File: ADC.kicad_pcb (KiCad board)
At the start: 2 copper layers, 199 parts, among them J1 Conn_01x03_Pin, J2 Screw_Terminal_01x02, J3 Screw_Terminal_01x09, SW1 SW_SPDT, U1 ADS1256IDBR, U10 CD4514BM, U11 ADG5412FBCPZ-RL7, U12 ADR421ARMZ, U13 OPA211ID, U14 ADG5412FBCPZ-RL7, U15 OPA211ID, U16 ADG5412FBCPZ-RL7, U17 OPA211ID, U18 CD4072BM, U19 CD4514BM, U2 MCU-STM32F407VET6_LQFP100_, U20 ADG5412FBCPZ-RL7, U21 ADG5412FBCPZ-RL7, U22 ADG5412FBCPZ-RL7, U23 ADG5412FBCPZ-RL7, U24 OPA211ID, U25 OPA211ID, U26 OPA211ID, U27 OPA211ID, U28 CD4043BPWR, U29 TLV1704AIPWR, U3 ADM2483xRW, U30 TLV1704AIPWR, U31 TLV1704AIPWR, U32 CD4072BM, U4 LM2596S-5, U5 DCP010505BP, U6 TLV1704AIPWR, U7 OPA211ID, U8 AMS1117-3.3, U9 ADG5412FBCPZ-RL7, Y1 8MHz, Y2 ABM3B-25.000MHZ-D2Y-T

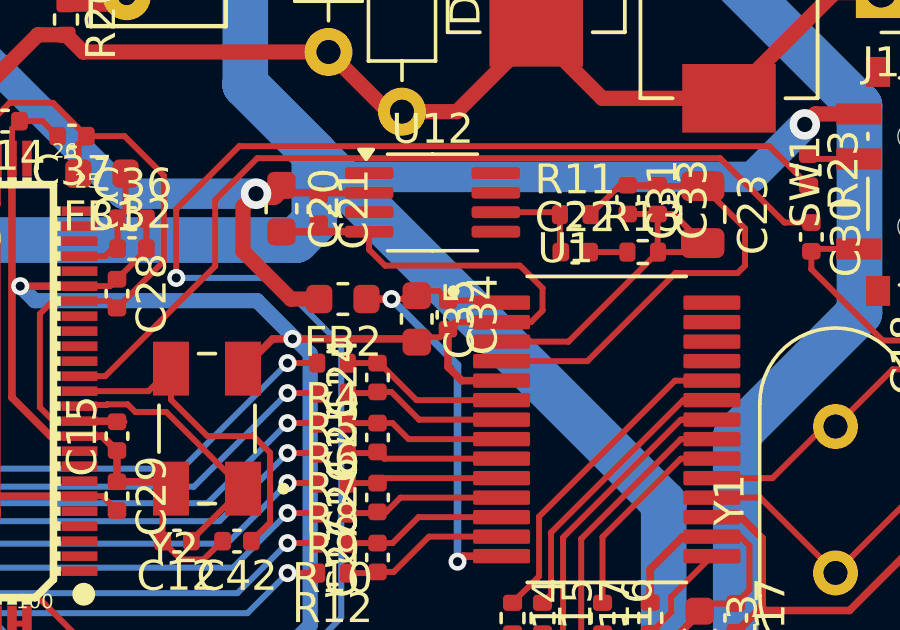
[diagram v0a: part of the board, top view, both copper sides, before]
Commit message: update
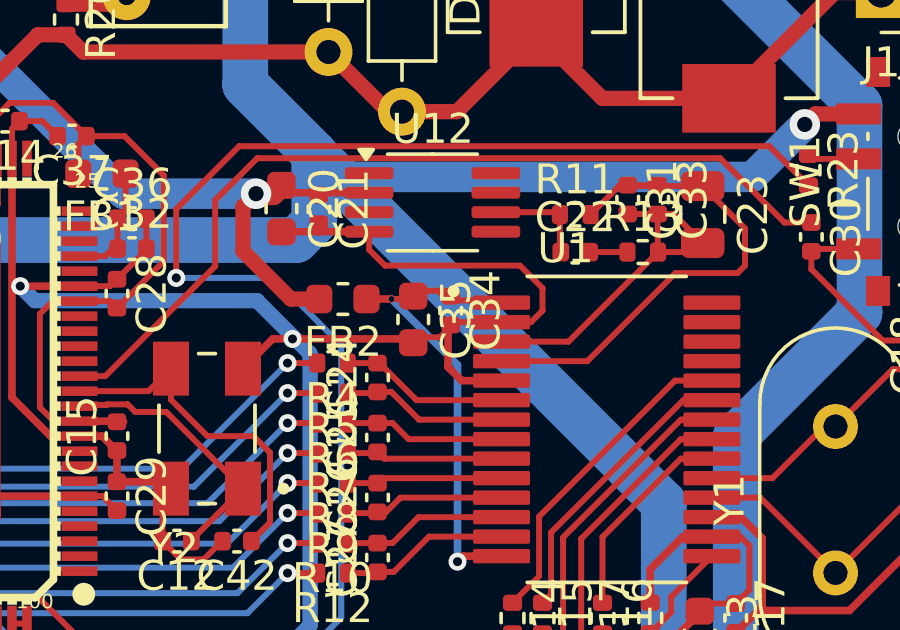
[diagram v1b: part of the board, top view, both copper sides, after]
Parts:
- moved C34 0.17 mm to (633.0, 474.1)
- moved C35 0.12 mm to (631.8, 474.4)
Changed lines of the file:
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@@
 		(tags "C Radial series Radial pin pitch 3.50mm diameter 8mm height 7mm Non-Polar Electrolytic Capacitor")
 		(property "Reference" "C4"
-			(at 1.75 -5.25 360)
+			(at 1.75 -5.25 0)
 			(layer "F.SilkS")
 			(effects
@@
 		)
 		(property "Value" "47uF"
-			(at 1.75 5.25 360)
+			(at 1.75 5.25 0)
 			(layer "F.Fab")
 			(effects
@@
 		)
 		(fp_text user "${REFERENCE}"
-			(at 1.75 0 360)
+			(at 1.75 0 0)
 			(layer "F.Fab")
 			(effects
@@
 		)
 		(fp_text user "${REFERENCE}"
-			(at 0 0 360)
+			(at 0 0 0)
 			(layer "F.Fab")
 			(effects
@@
 		(tags "C Radial series Radial pin pitch 3.50mm diameter 8mm height 7mm Non-Polar Electrolytic Capacitor")
 		(property "Reference" "C1"
-			(at 1.75 -5.25 360)
+			(at 1.75 -5.25 0)
 			(layer "F.SilkS")
 			(effects
@@
 		)
 		(property "Value" "47uF"
-			(at 1.75 5.25 360)
+			(at 1.75 5.25 0)
 			(layer "F.Fab")
 			(effects
@@
 		)
 		(fp_text user "${REFERENCE}"
-			(at 1.75 0 360)
+			(at 1.75 0 0)
 			(layer "F.Fab")
 			(effects
@@
 	(footprint "Capacitor_SMD:C_0402_1005Metric"
 		(layer "F.Cu")
-		(at 632.959137 474.220735 -90)
+		(at 633.05 474.08 -90)
 		(descr "Capacitor SMD 0402 (1005 Metric), square (rectangular) end terminal, IPC_7351 nominal, (Body size source: IPC-SM-782 page 76, https://www.pcb-3d.com/wordpress/wp-content/uploads/ipc-sm-782a_amendment_1_and_2.pdf), generated with kicad-footprint-generator")
 		(tags "capacitor")
@@
 		(at 596.075 439.91 180)
 		(property "Reference" "U5"
-			(at -3.30232 -19.4583 360)
+			(at -3.30232 -19.4583 0)
 			(layer "F.SilkS")
 			(effects
@@
 		)
 		(property "Value" "DCP010505BP"
-			(at 10.445985 4.041125 360)
+			(at 10.445985 4.041125 0)
 			(layer "F.Fab")
 			(effects
@@
 		)
 		(property "Footprint" "DCP10505BP:DIP254P762X533-7P"
-			(at 0 0 360)
+			(at 0 0 0)
 			(layer "F.Fab")
 			(hide yes)
@@
 		)
 		(property "Datasheet" ""
-			(at 0 0 360)
+			(at 0 0 0)
 			(layer "F.Fab")
 			(hide yes)
@@
 		)
 		(property "Description" ""
-			(at 0 0 360)
+			(at 0 0 0)
 			(layer "F.Fab")
 			(hide yes)
@@
 	(footprint "Capacitor_SMD:C_0603_1608Metric"
 		(layer "F.Cu")
-		(at 631.916637 474.358235 -90)
+		(at 631.8 474.375 -90)
 		(descr "Capacitor SMD 0603 (1608 Metric), square (rectangular) end terminal, IPC_7351 nominal, (Body size source: IPC-SM-782 page 76, https://www.pcb-3d.com/wordpress/wp-content/uploads/ipc-sm-782a_amendment_1_and_2.pdf), generated with kicad-footprint-generator")
 		(tags "capacitor")
@@
 	(via
 		(at 631.075 473.695735)
-		(size 0.6)
-		(drill 0.3)
+		(size 0.2)
+		(drill 0.2)
 		(layers "F.Cu" "B.Cu")
 		(net 25)
